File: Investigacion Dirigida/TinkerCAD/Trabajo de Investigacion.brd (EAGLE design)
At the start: 176.8 x 266 mm, 10 parts, among them P1 BATTERYGENERIC, U1 OPAMP_DIP, U2 ARDUINO-UNO-R3-SHIELD, U4 LCD-16X2JHD-162A

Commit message: update
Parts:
- removed R3: 220, Tinkercad:RESAD1016W63L850D250B
- removed RPOT2: 10k, Tinkercad:HA-06-SM065
- removed S1: TOGGLE, Tinkercad:SWITCH-SPDT-PTH-8.5X3.7MM
- removed U4: LCD-16X2JHD-162A, Tinkercad:JHD-162A
- added U3: LCD-16X2-I2CSUNFOUNDER-IIC, Tinkercad:LCD-I2C
- moved U2 172.0 mm to (89.8, 68.7)
- moved U1 103.8 mm to (127.5, 10.2)
- moved R1 103.8 mm to (95.8, 16.6)
- moved R2 103.8 mm to (100.8, 8.97)
- moved RPOT1 103.8 mm to (80.5, 21.7)
- moved P1 102.5 mm to (8.26, 40.5)
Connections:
- removed net U2_D2: U2.D2, U4.4
- removed net U2_D3: U2.D3, U4.6
- removed net U2_D4: U2.D4, U4.11
- removed net U2_D5: U2.D5, U4.12
- removed net U2_D6: U2.D6, U4.13
- removed net U2_D7: U2.D7, U4.14
- removed net U4_LED+: R3.1, U4.15
- removed net U4_VO: RPOT2.2, U4.3
- new net U2_SCL: U2.SCL, U3.4
- new net U2_SDA: U2.SDA, U3.3
- net P1-: now also U3.1; no longer RPOT2.3, U4.1, U4.16, U4.5
- net U2_5V: now also U3.2; no longer R3.2, RPOT2.1, U4.2
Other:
- board size 176.8 x 266 mm -> 223.3 x 98.5 mm

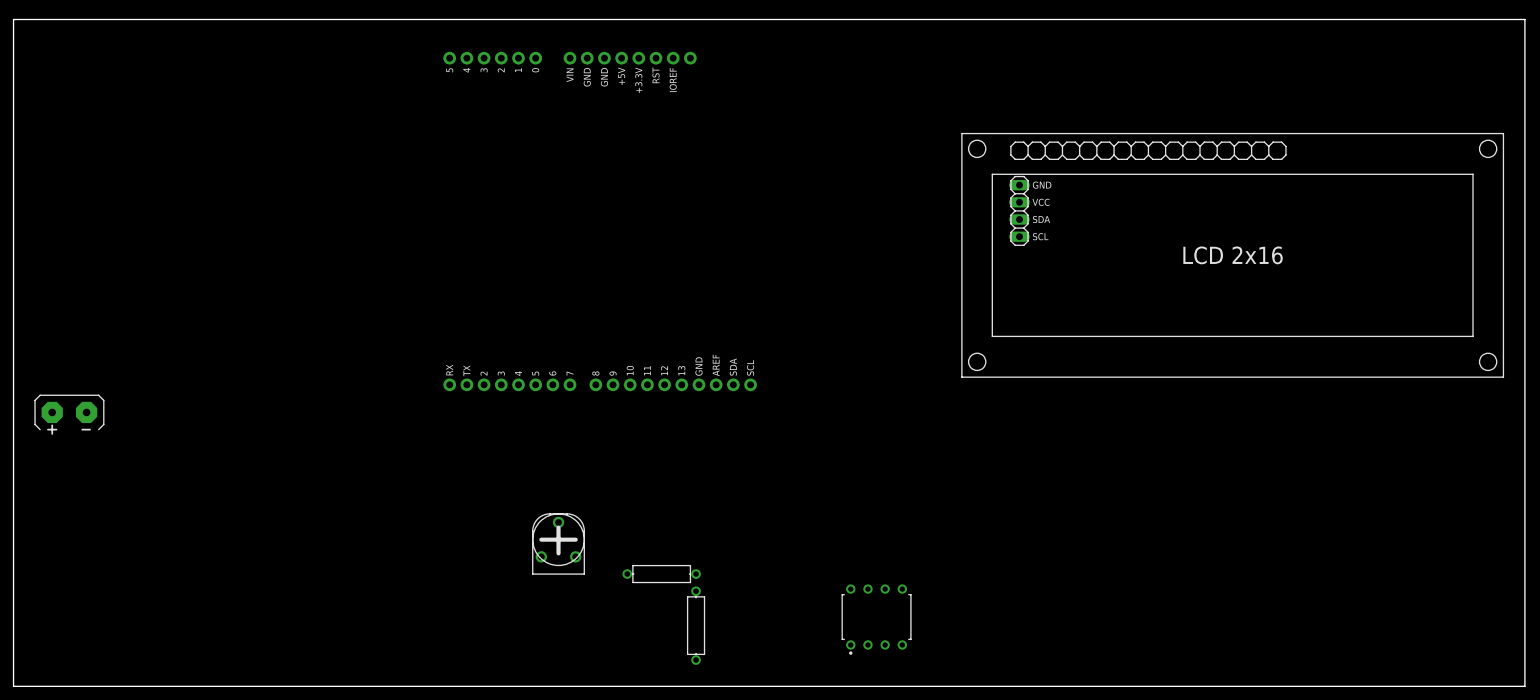
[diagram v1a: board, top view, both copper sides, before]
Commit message: Ultimos cambios
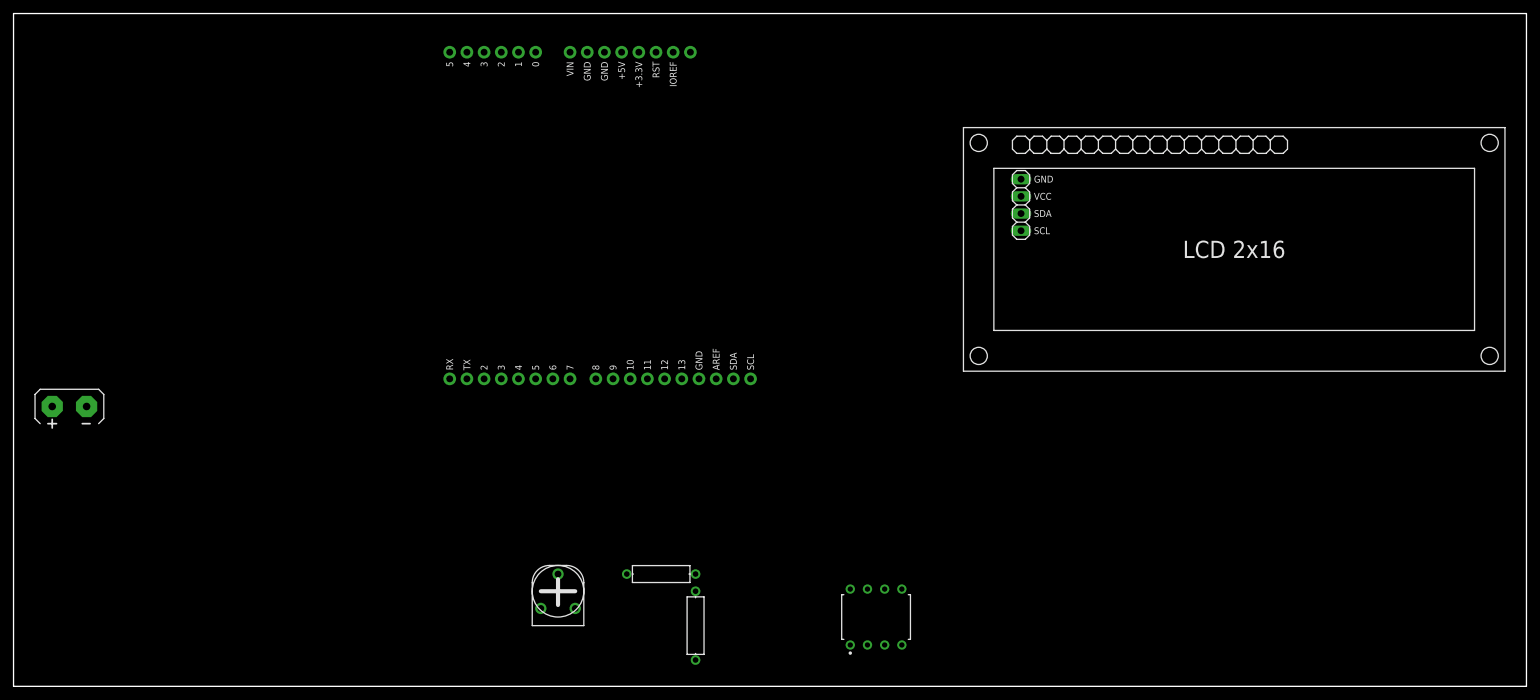
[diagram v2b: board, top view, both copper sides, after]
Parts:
- moved RPOT1 7.62 mm to (80.4, 14.1)
- moved U3 0.91 mm to (167.9, 80.0)
- moved U2 0.88 mm to (89.8, 69.6)
- moved P1 0.88 mm to (8.26, 41.3)
- moved R1 0.07 mm to (95.7, 16.6)
- moved R2 0.07 mm to (100.8, 8.97)
- moved U1 0.07 mm to (127.4, 10.2)
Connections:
- removed net U2_SCL: U2.SCL, U3.4
- removed net U2_SDA: U2.SDA, U3.3
- new net U2_A4: U2.A4, U3.3
- new net U2_A5: U2.A5, U3.4
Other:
- board size 223.3 x 98.5 mm -> 223.5 x 99.4 mm
